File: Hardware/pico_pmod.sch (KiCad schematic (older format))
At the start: 8 parts, among them J1 Conn_02x15_Odd_Even, J2 Conn_01x02, J3 Conn_01x02, J4 Conn_01x02, J5 Conn_01x03, J6 Conn_01x02, U1 Pico

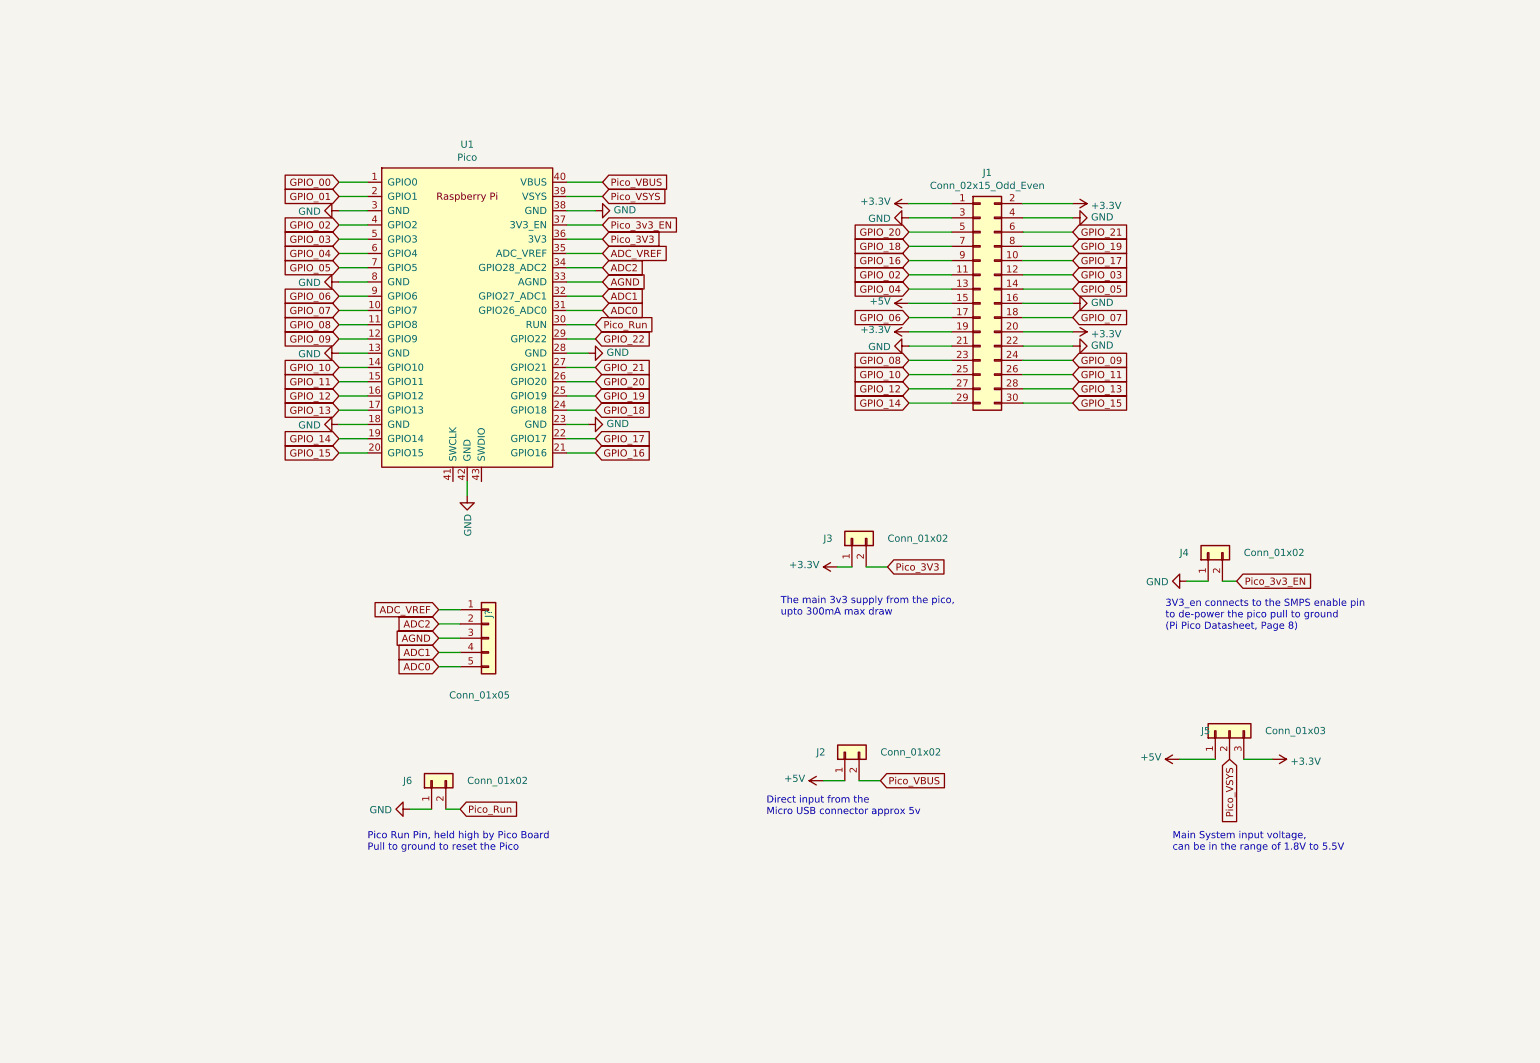
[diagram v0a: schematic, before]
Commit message: Minor circuit changes
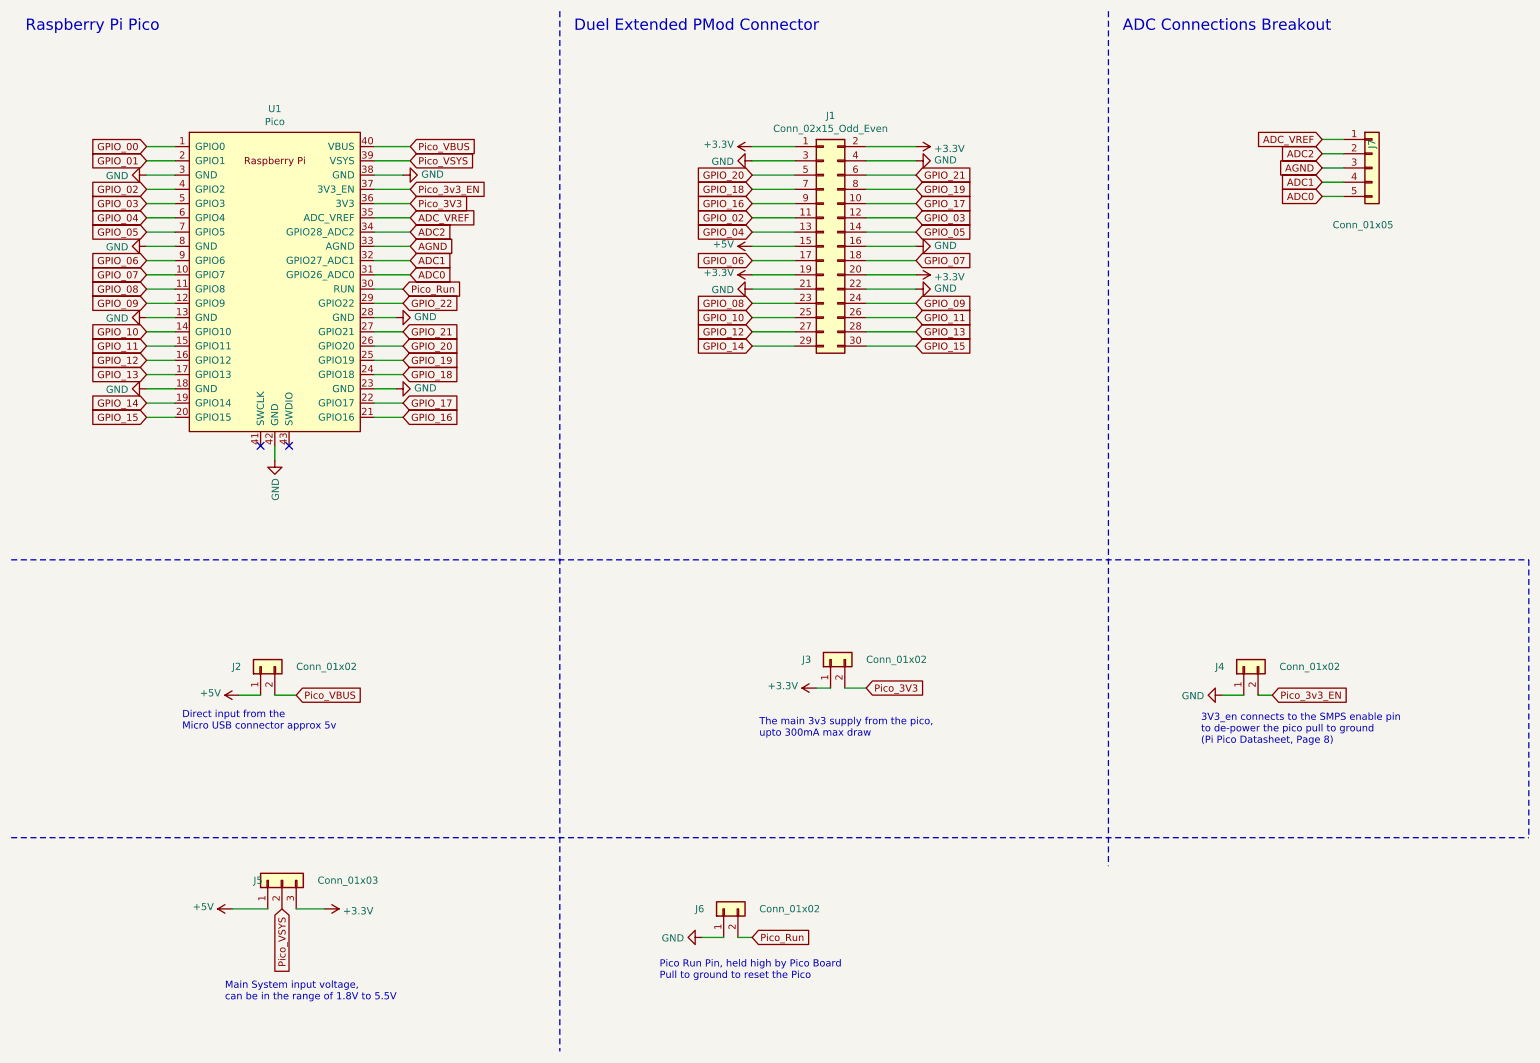
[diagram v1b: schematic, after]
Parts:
- gave numbers to parts that had none: 1
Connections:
- no-connect marks 0 -> 2
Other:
- note added: "ADC Connections Breakout\n"
- note added: "Duel Extended PMod Connector"
- note added: "Raspberry Pi Pico"
- moved on the sheet: J1, J2, J3, J4, J5, J6, J7, U1
